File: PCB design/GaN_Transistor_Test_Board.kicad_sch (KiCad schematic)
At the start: 4 parts, among them Q1 IGD70R500D2S

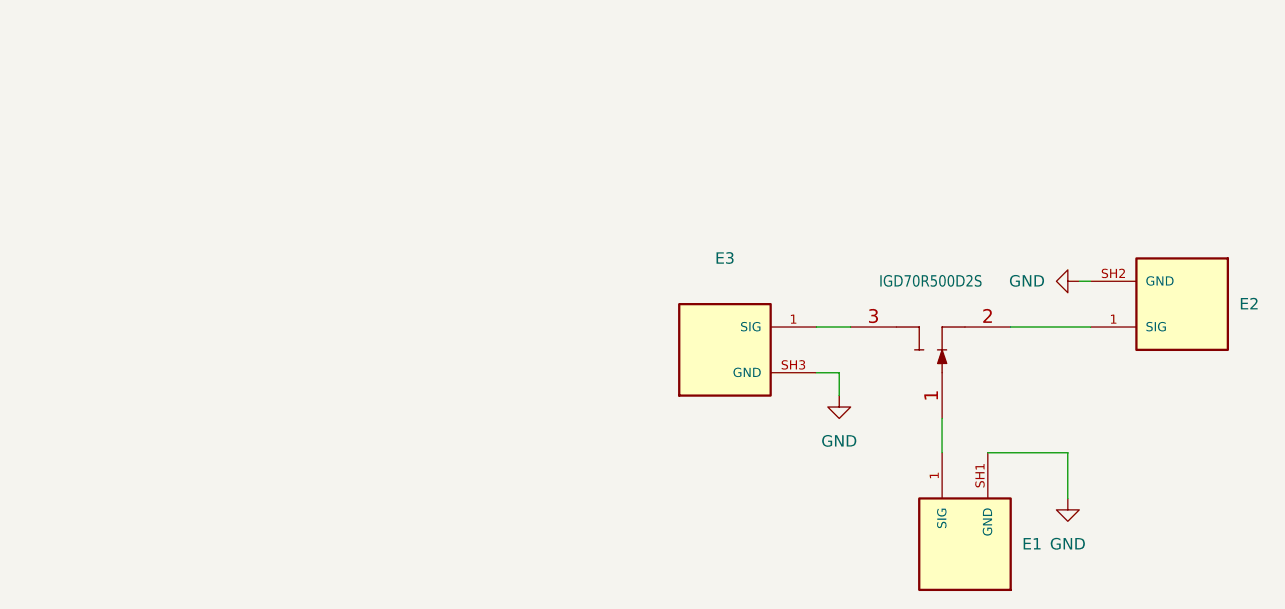
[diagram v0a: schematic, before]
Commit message: Layout redesign
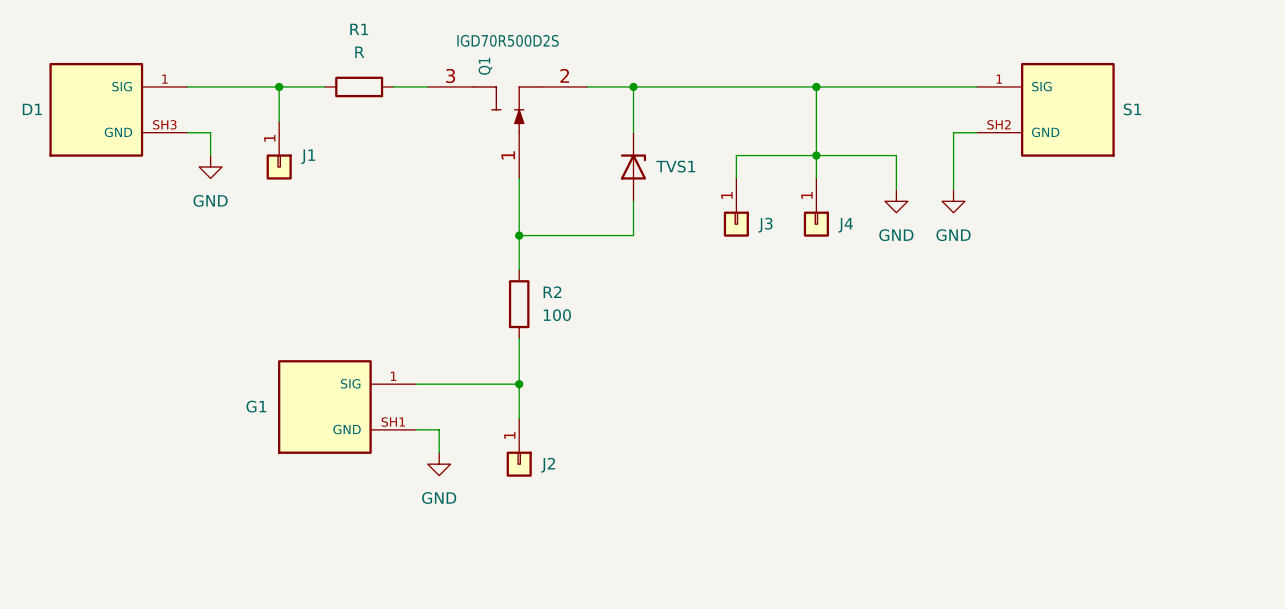
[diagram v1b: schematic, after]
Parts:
- added J1, J2, J3, J4: Conn_01x01, symbol Connector_Generic:Conn_01x01
- added R1: R, Resistor_SMD:R_0805_2012Metric_Pad1.20x1.40mm_HandSolder, symbol Device:R
- added R2: 100, Resistor_SMD:R_0805_2012Metric_Pad1.20x1.40mm_HandSolder, symbol Device:R
- added TVS1: D_Zener, Footprints:SMFSeries_LTF, symbol Device:D_Zener
- Q1: footprint Footprints:TO-252-3_TabPin4 -> Footprints:IFX-PG-TO252-3N-37-V1
- renumbered E3 to D1, E1 to G1, E2 to S1
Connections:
- net GND: now also Q1.2 (S), S1.1 (SIG), J3.1 (Pin_1), J4.1 (Pin_1), TVS1.1 (K)
- net at Q1.1 (G): now also R2.1, TVS1.2 (A); no longer G1.1 (SIG)
- net at D1.1 (SIG): now also J1.1 (Pin_1), R1.1; no longer Q1.3 (D)
- new net: G1.1 (SIG), J2.1 (Pin_1), R2.2
- new net: Q1.3 (D), R1.2
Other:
- company: (none) -> eng. Mateusz Witczak
- title: (none) -> GaN Transistor Test Board
- moved on the sheet: D1, G1, S1
